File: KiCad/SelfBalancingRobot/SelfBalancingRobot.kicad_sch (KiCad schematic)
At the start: 16 parts, among them U1 ESP32_NODEMCU, U8 L7805

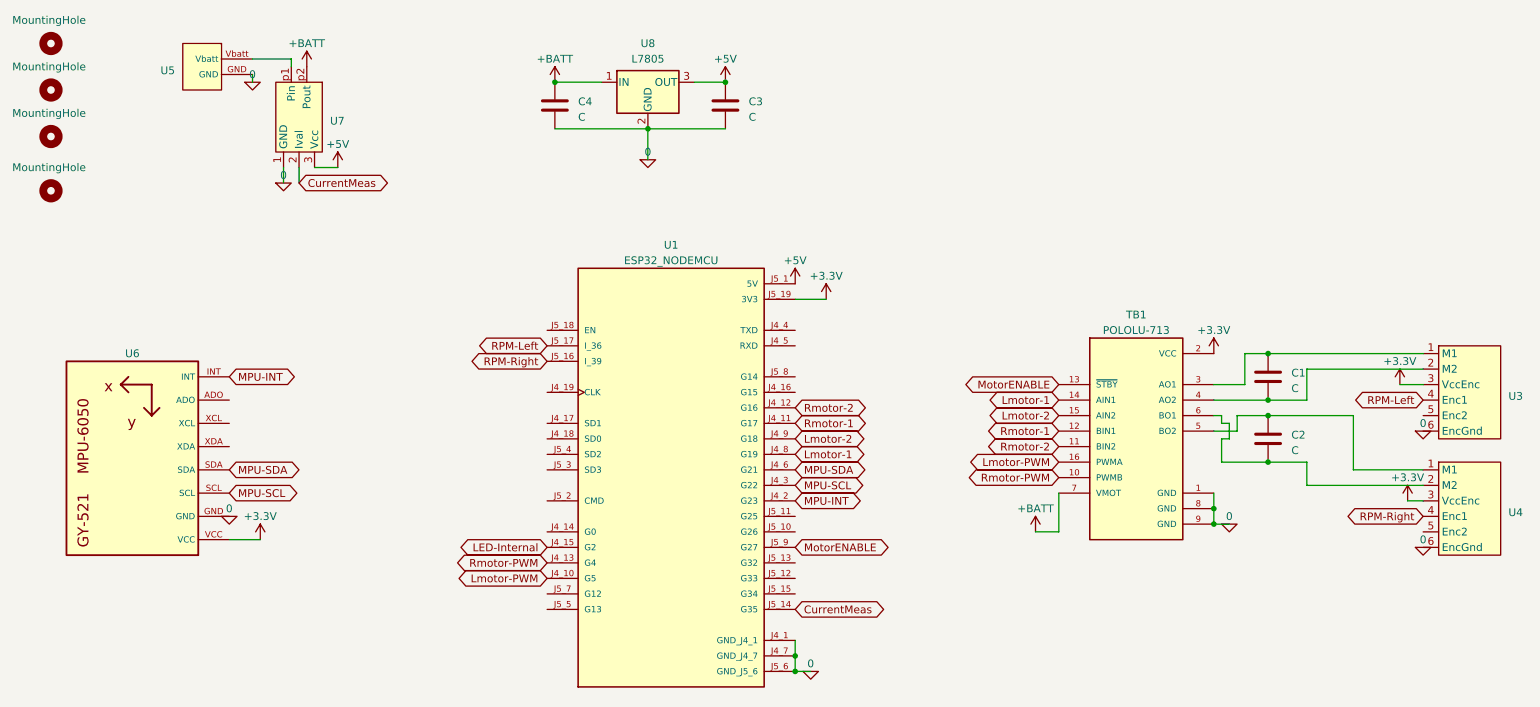
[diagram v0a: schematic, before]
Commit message: kicad done and pid integrated
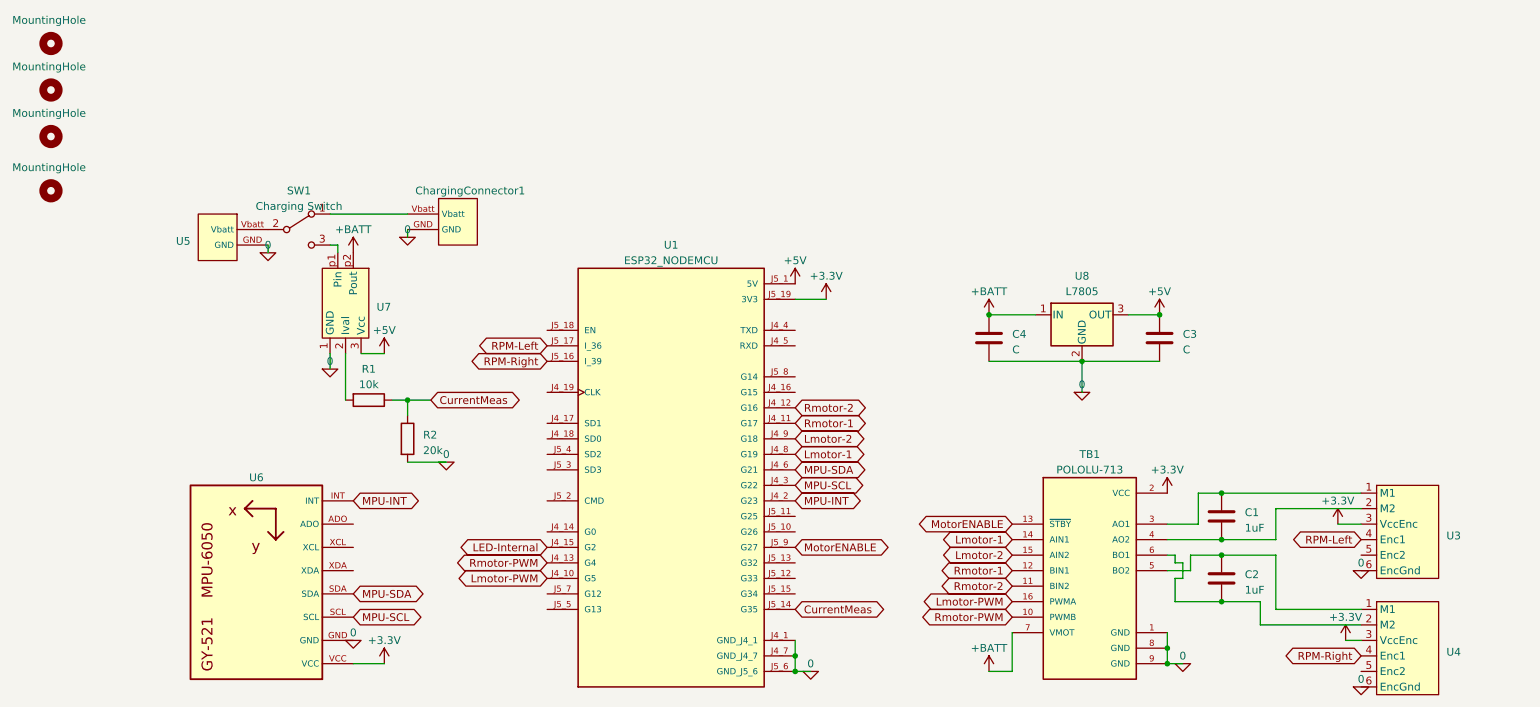
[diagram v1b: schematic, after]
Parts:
- added ChargingConnector1: ~, 0_Footprints:ChargingConnector, symbol 0_Library:BatteryConnector
- added R1: 10k, Resistor_THT:R_Axial_DIN0207_L6.3mm_D2.5mm_P7.62mm_Horizontal, symbol Device:R
- added R2: 20k, Resistor_THT:R_Axial_DIN0207_L6.3mm_D2.5mm_P7.62mm_Horizontal, symbol Device:R
- added SW1: Charging Switch, Connector_Phoenix_MSTB:PhoenixContact_MSTBA_2,5_3-G-5,08_1x03_P5.08mm_Horizontal, symbol Switch:SW_SPDT
- C1, C2: value C -> 1uF
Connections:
- net 0: now also ChargingConnector1.GND, R2.2
- net CurrentMeas: now also R1.1, R2.1; no longer U7.2 (Ival)
- net at U5.Vbatt: now also SW1.2 (B); no longer U7.p1 (Pin)
- new net: R1.2, U7.2 (Ival)
- new net: ChargingConnector1.Vbatt, SW1.1 (A)
- new net: SW1.3 (C), U7.p1 (Pin)
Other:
- moved on the sheet: C1, C2, C3, C4, TB1, U3, U4, U5, U6, U7, U8
